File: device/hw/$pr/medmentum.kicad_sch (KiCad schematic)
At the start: 135 parts, among them CON1 ZX-IDC2.54-2-13PZZ, J1 Conn_01x01_Pin, J2 Conn_01x01_Pin, J3 Conn_01x01_Pin, J4 Conn_01x01_Pin, J5 Conn_01x01_Pin, Q1 PNP, Q2 NPN, Q3 NPN, SW1 SW_SPDT, SW2 SW_SPDT, SW3 SW_Push, SW4 SW_Push, SW5 SW_SPDT, U1 TPS62082DSGR, U2 BQ27441DRZR-G1B, U3 USBLC6-2SC6, U4 BQ24074RGTR, U5 TS3USB221ARSER, U6 TPS63002DRCT, U7 STM32F411CEU6, U8 ESP32-C3-MINI-1-H4, Y1 12.5pF, Y2 18pF

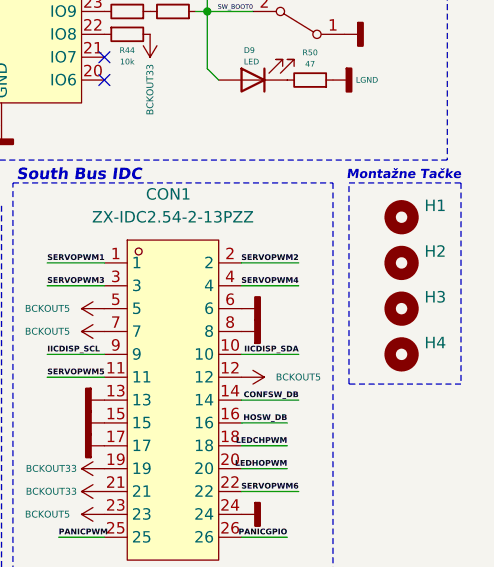
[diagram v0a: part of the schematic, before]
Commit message: application
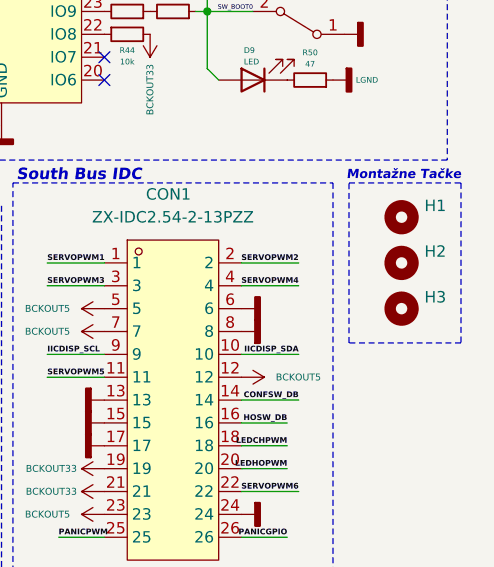
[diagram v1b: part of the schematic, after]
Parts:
- removed H4: ~, MountingHole:MountingHole_2.5mm, symbol Mechanical:MountingHole
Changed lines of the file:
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@@
 	(rectangle
 		(start 269.748 66.04)
-		(end 282.194 88.392)
+		(end 282.194 83.82)
 		(stroke
 			(width 0)
@@
 					(unit 1)
 				)
-			)
-		)
-	)
-	(symbol
-		(lib_id "Mechanical:MountingHole")
-		(at 275.59 85.09 0)
-		(unit 1)
-		(exclude_from_sim yes)
-		(in_bom no)
-		(on_board yes)
-		(dnp no)
-		(fields_autoplaced yes)
-		(property "Reference" "H4"
-			(at 278.13 83.8199 0)
-			(effects
-				(font
-					(size 1.27 1.27)
-				)
-				(justify left)
-			)
-		)
-		(property "Value" "~"
-			(at 278.13 86.3599 0)
-			(effects
-				(font
-					(size 1.27 1.27)
-				)
-				(justify left)
-			)
-		)
-		(property "Footprint" "MountingHole:MountingHole_2.5mm"
-			(at 275.59 85.09 0)
-			(effects
-				(font
-					(size 1.27 1.27)
-				)
-				(hide yes)
-			)
-		)
-		(property "Datasheet" "~"
-			(at 275.59 85.09 0)
-			(effects
-				(font
-					(size 1.27 1.27)
-				)
-				(hide yes)
-			)
-		)
-		(property "Description" "Mounting Hole without connection"
-			(at 275.59 85.09 0)
-			(effects
-				(font
-					(size 1.27 1.27)
-				)
-				(hide yes)
-			)
-		)
-		(instances
-			(project "medmentum"
-				(path "/ead52261-b3da-41ef-908f-3daaabe10954"
-					(reference "H4")
-					(unit 1)
-				)
